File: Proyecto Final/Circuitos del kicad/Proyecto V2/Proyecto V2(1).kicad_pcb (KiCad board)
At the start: 2 copper layers, 259.7 x 176.3 mm, 44 parts, among them J1 12v, J2 I2C + LCD, J3 DS1307, Q1 PN2222A, Q2 PN2222A, Q3 PN2222A, SW1 SW_Push, SW2 SW_Push, SW3 SW_Push, SW4 SW_Push, U1 LM7805, U3 ATmega328P-P, Y1 16MHz

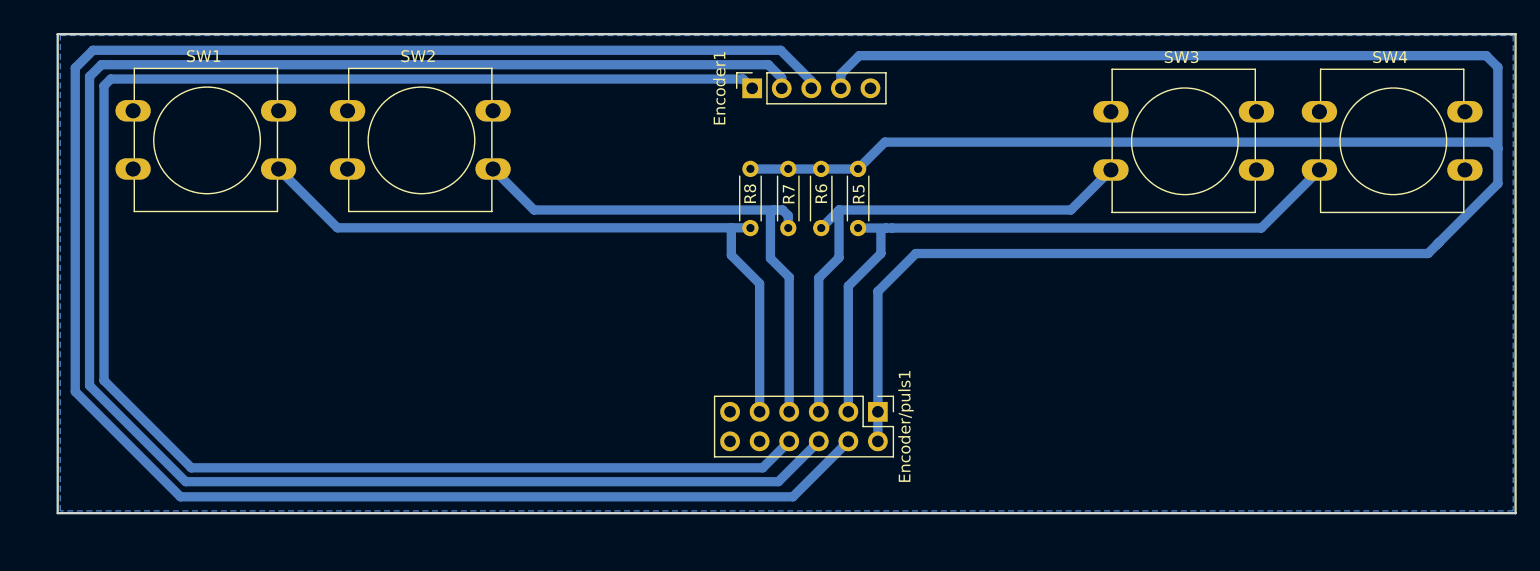
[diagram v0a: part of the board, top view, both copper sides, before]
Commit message: Cambios generales
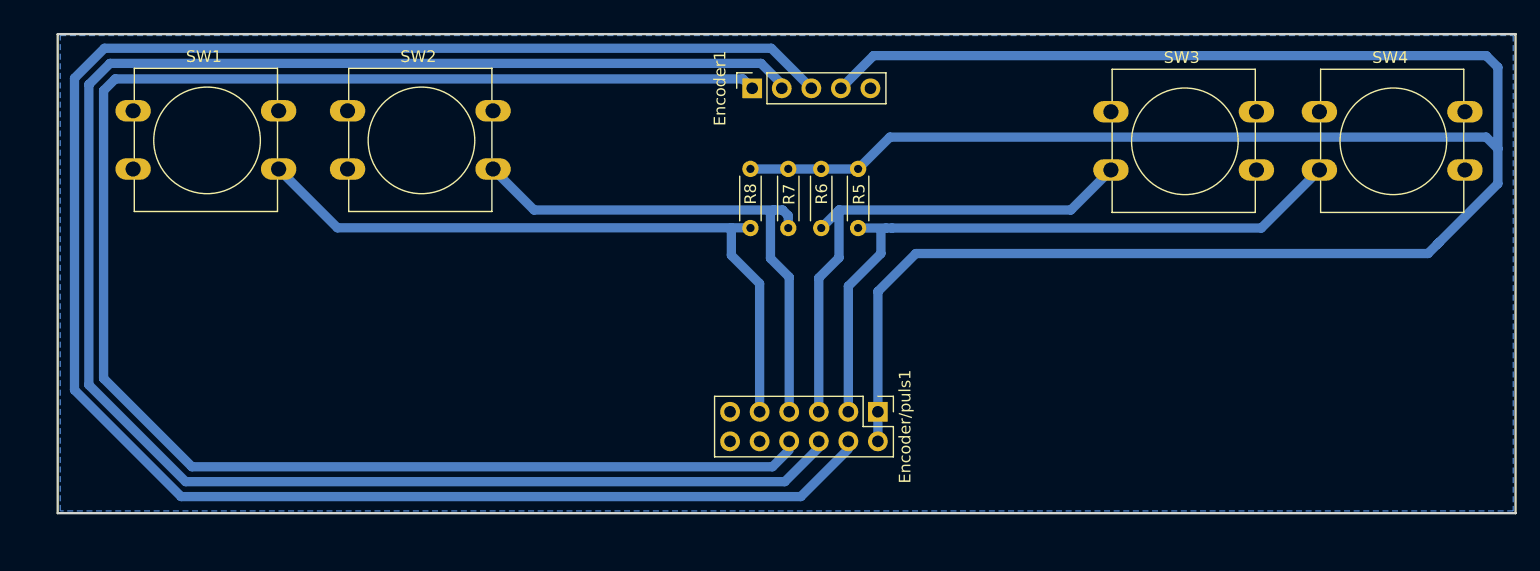
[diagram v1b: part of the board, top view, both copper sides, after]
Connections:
- Encoder1 pad 1: Net-(Encoder/puls1-Pad8) -> Net-(Encoder/puls1-Pad4)
- Encoder1 pad 3: Net-(Encoder/puls1-Pad4) -> Net-(Encoder/puls1-Pad8)
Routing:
- net Net-(Encoder/puls1-Pad4): track 165.5 -> 164.5 mm
- net Net-(Encoder/puls1-Pad6): track 155.3 -> 154.5 mm
- net Net-(Encoder/puls1-Pad8): track 144.5 -> 143.8 mm
